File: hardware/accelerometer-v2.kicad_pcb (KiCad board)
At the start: 2 copper layers, 20 x 25 mm, 25 parts, among them P1 CON-SENSOR, P2 Debug, P3 Boot, U1 XMC1100, U2 KX122-1037, U3 DRILL, U4 DRILL, U5 DRILL, U6 DRILL

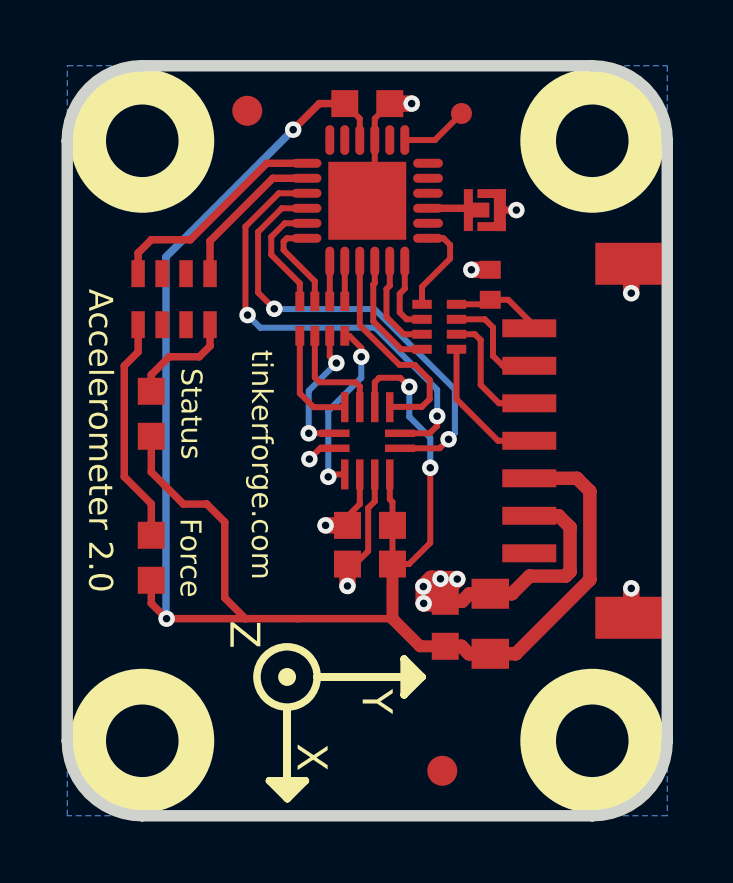
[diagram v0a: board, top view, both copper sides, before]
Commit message: Fix origin
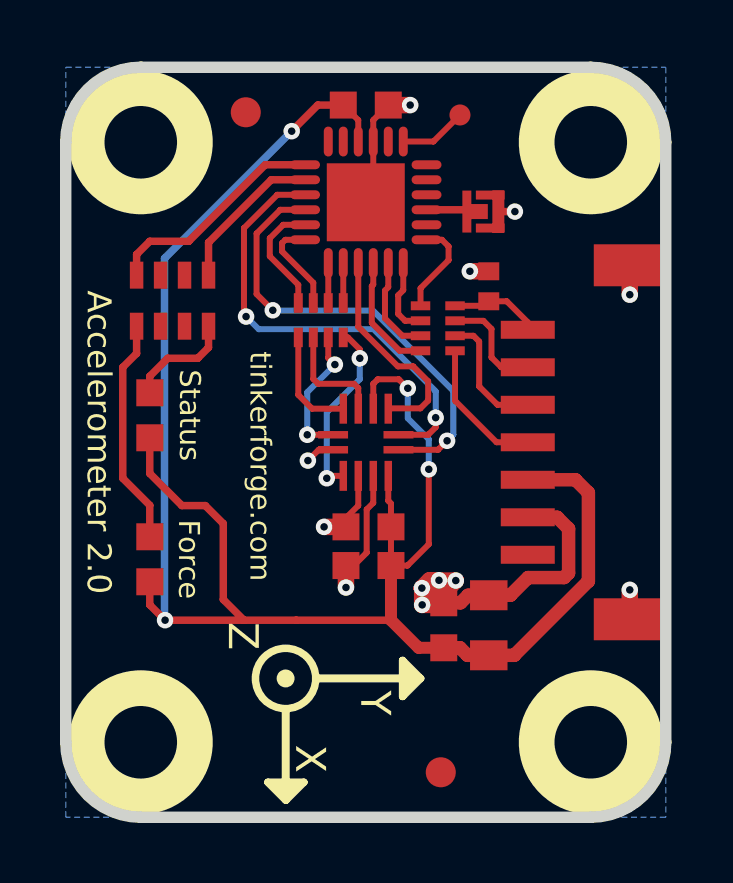
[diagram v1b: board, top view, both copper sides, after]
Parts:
- moved P2 0.07 mm to (134.6, 89.3)
- moved P3 0.07 mm to (135.4, 92.5)
- moved C1 0.07 mm to (135.6, 95.0)
- moved C2 0.07 mm to (135.6, 106.3)
- moved C3 0.07 mm to (134.1, 106.3)
- moved C4 0.07 mm to (131.5, 89.0)
- moved Fiducial_Mark 0.07 mm to (134.0, 111.2)
- moved G*** 0.07 mm to (131.5, 100.2)
- moved P1 0.07 mm to (141.5, 100.2)
- moved RP2 0.07 mm to (130.0, 96.1)
- moved U1 0.07 mm to (131.5, 92.2)
- moved U2 0.07 mm to (131.5, 100.2)
- moved VAL 0.07 mm to (131.5, 92.2)
- moved VAL 0.07 mm to (131.5, 108.2)
- moved D1 0.07 mm to (124.3, 99.3)
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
